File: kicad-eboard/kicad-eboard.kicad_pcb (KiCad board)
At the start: 2 copper layers, 93 parts, among them J1 Conn_02x03, J2 Conn_01x02, J3 Conn_01x10, M1 Hopper_Servo, SW1 LIMIT_1, SW2 LIMIT_2, SW3 SRX_Encoder, U1 TinkerBoard, U10 REF2033, U11 PDQ15-Q24-S12-D, U12 PDQ30-Q24-S5-D, U13 Hokuyo_UST-10LX, U14 Hokuyo_UST-10LX, U15 MPU-6050, U2 Sabertooth2x60, U3 Sabertooth2x60, U4 Sabertooth2x60, U5 Sabertooth2x60, U6 INA4181, U7 INA4181, U8 ADS1015IDGS, U9 MCP3008

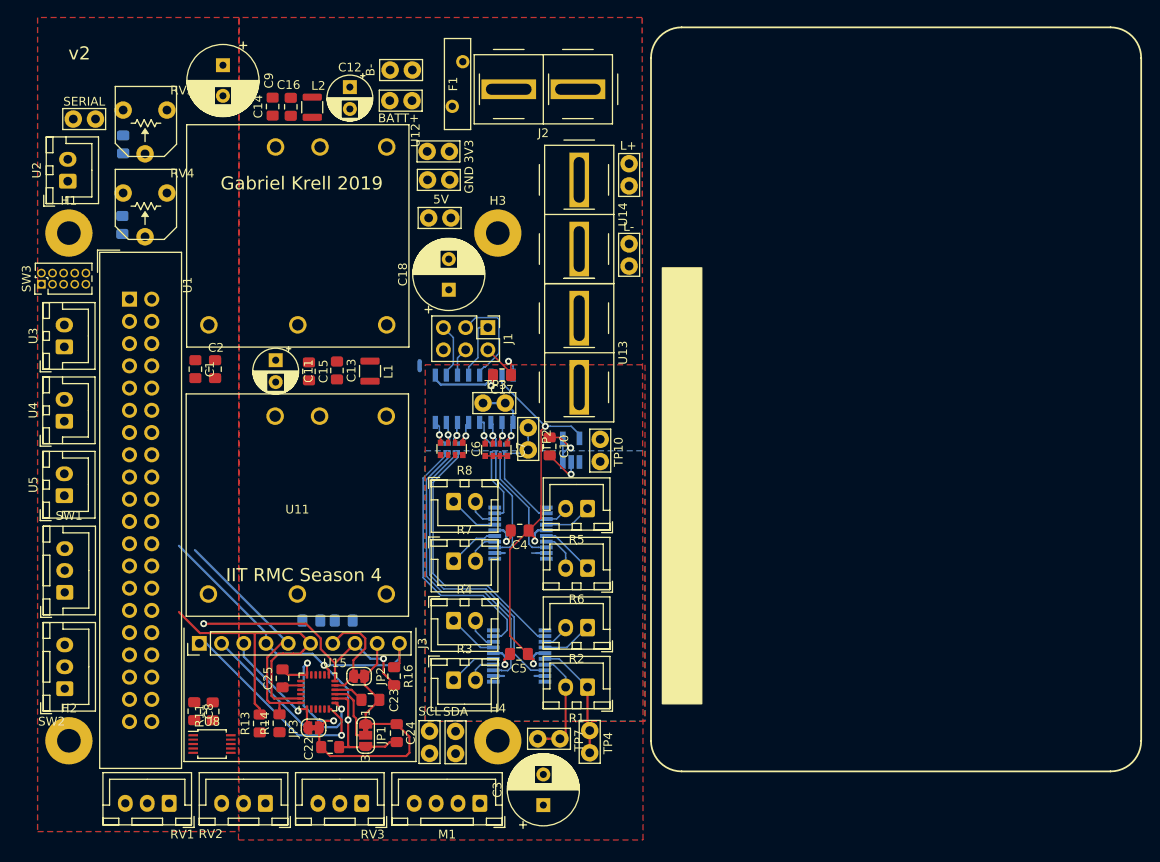
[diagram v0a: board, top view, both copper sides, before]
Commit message: Finish routing?
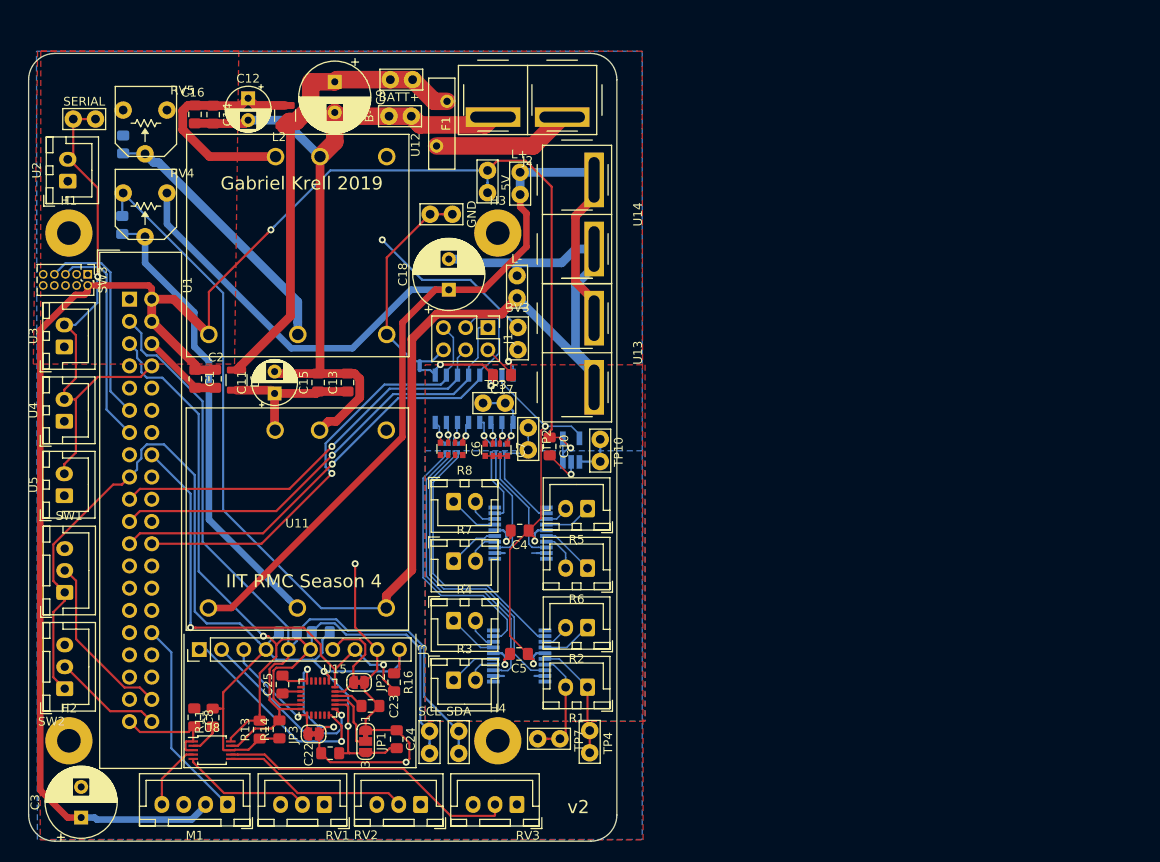
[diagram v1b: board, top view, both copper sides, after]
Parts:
- moved C3 52.8 mm to (29.8, 103.7)
- moved M1 28.8 mm to (46.5, 102.2)
- moved TP15 21.6 mm to (79.7, 47.7), turned to 270 degrees
- moved RV1 17.7 mm to (57.6, 102.2)
- moved RV2 17.7 mm to (68.6, 102.2)
- moved RV3 17.7 mm to (79.6, 102.2)
- moved L1 15.3 mm to (47.5, 54.8)
- moved TP12 13.3 mm to (79.6, 41.8)
- moved C9 12.9 mm to (58.8, 19.6)
- moved TP11 12.5 mm to (80.0, 32.5)
- moved C12 11.7 mm to (48.9, 21.5)
- moved C16 11.0 mm to (42.8, 23.4)
- moved TP13 8.64 mm to (76.2, 29.8), turned to 270 degrees
- moved C14 6.86 mm to (44.9, 23.4), turned to 270 degrees
- moved SW3 5.41 mm to (30.6, 41.6), turned to 270 degrees
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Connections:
- U1 pad 16: Net-(U1-Pad16) -> /IMU/INT
- U1 pad 27: /IMU/INT -> Net-(U1-Pad27)
- U8 pad 4: Net-(RV1-Pad2) -> Net-(M1-Pad4)
- U8 pad 5: Net-(RV2-Pad2) -> Net-(RV1-Pad2)
- U8 pad 6: Net-(RV3-Pad2) -> Net-(RV2-Pad2)
- U8 pad 7: Net-(M1-Pad4) -> Net-(RV3-Pad2)
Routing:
- net +5V: track 9.19 -> 202.8 mm, vias 1 -> 2
- net GNDA: track 0.00 -> 163.3 mm
- net +12V: track 0.00 -> 140.7 mm
- net +3V3: track 67.0 -> 188.9 mm, vias 3 -> 4
- net GND: track 47.1 -> 133.5 mm, vias 2 -> 4
- net GNDPWR: track 0.00 -> 84.2 mm
- net /SDA: track 28.3 -> 97.5 mm
- net /SCL: track 38.8 -> 101.6 mm, vias 0 -> 1
- net Net-(TP1-Pad1): track 0.00 -> 60.6 mm, vias 0 -> 1
- net +BATT: track 0.00 -> 54.1 mm
- net Net-(C20-Pad1): track 0.00 -> 52.4 mm
- net /SCLK: track 11.7 -> 60.0 mm, vias 0 -> 1
- net /MISO: track 6.95 -> 52.9 mm, vias 0 -> 1
- net /SS: track 6.24 -> 51.2 mm, vias 0 -> 1
- net /MOSI: track 3.28 -> 46.9 mm, vias 0 -> 1
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- added copper zone on B.Cu, net GND
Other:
- board outline added: 67.2 x 90 mm
- copper layers 2 -> 4
